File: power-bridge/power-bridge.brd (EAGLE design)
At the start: 9.8 x 22.4 mm, 3 parts, among them X2 CON-MA03-2PCB_EDGE

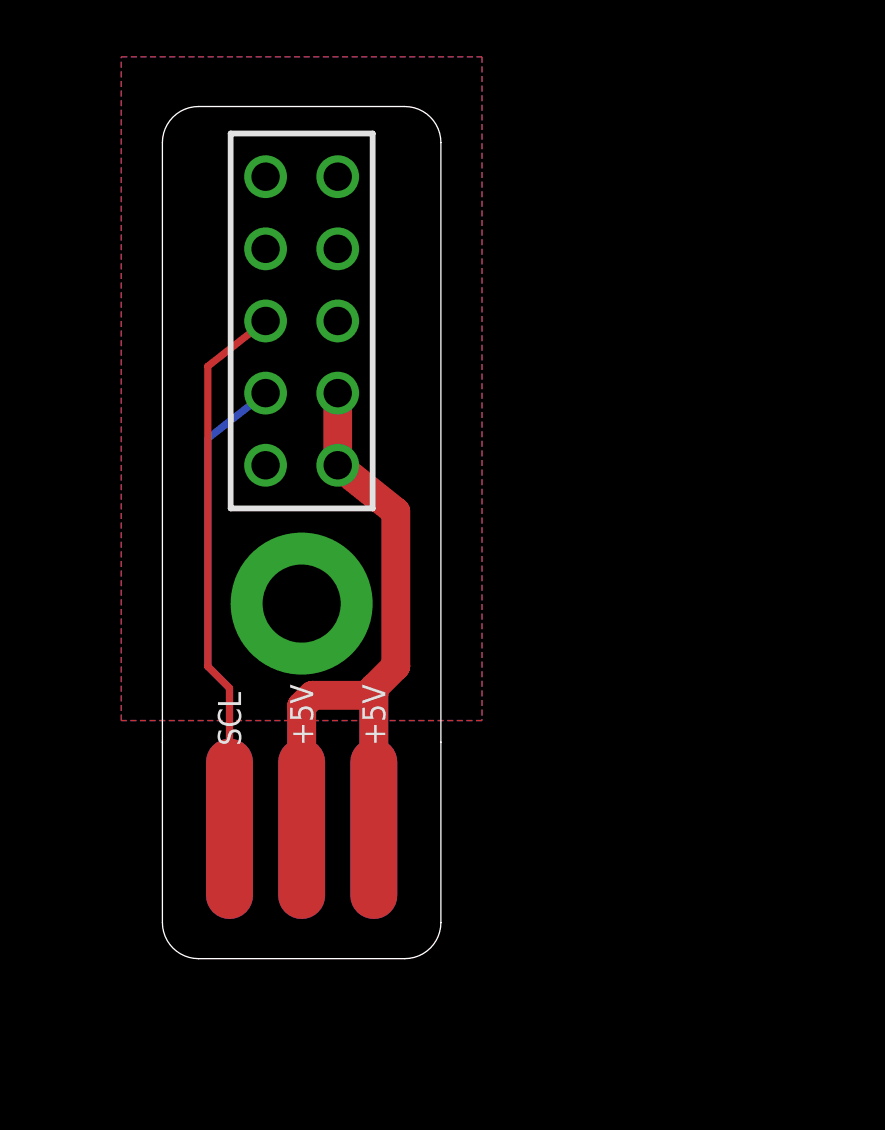
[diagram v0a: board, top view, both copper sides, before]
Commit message: Publish v1.0.0 Power Board and Power Bridge
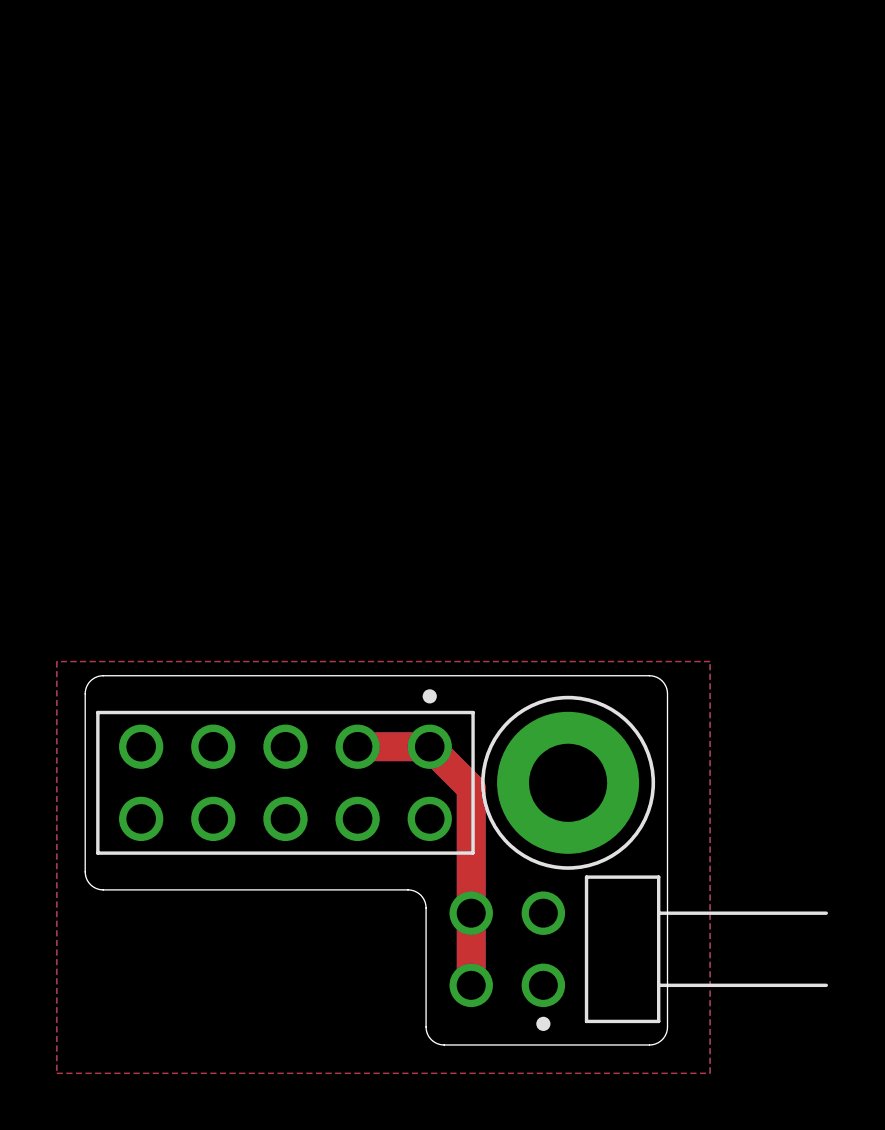
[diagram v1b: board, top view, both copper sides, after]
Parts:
- removed U$2: MOUNTINGHOLE2.7_THICK, sanisimov:MOUNTINGHOLE_2.7_PLATED_THICK
- added U$1: MOUNTINGHOLE2.7_THICK, _Library.b1f76137-4d0f-4ce2-9703-0cd83550450f.flbr:MOUNTINGHOLE_2.7_PLATED_THICK
- X1: value (none) -> CON-MA02-2; device sanisimov:FE05-2 -> _Library.b1f76137-4d0f-4ce2-9703-0cd83550450f.flbr:HDRRA4W64P254_2X2_508X254X556B
- X2: value CON-MA03-2PCB_EDGE -> CON-FE05-2; device sanisimov:PCB_EDGE_03-2 -> _Library.b1f76137-4d0f-4ce2-9703-0cd83550450f.flbr:HDRVR10W64P254_2X5_1270X508X850B
- moved X1 24.9 mm to (16.1, 1.60)
- moved X2 8.72 mm to (12.1, 10.0), turned to 180 degrees
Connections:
- removed net N$1: X1.3, X2.4
- removed net N$2: X1.5, X2.1
- removed net PWR: X1.2, X1.4, X2.2, X2.3
- new net +5V: X1.2, X1.4, X2.1, X2.3
- net GND: now also X1.1, X1.3, X2.10; no longer X1.6, X1.9, X2.6
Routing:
- net PWR: track 23.7 -> 0.00 mm
- net +5V: track 0.00 -> 23.1 mm
- net N$2: track 19.2 -> 0.00 mm
- net N$1: track 16.6 -> 0.00 mm
- net GND: track 9.27 -> 0.00 mm
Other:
- board size 9.8 x 22.4 mm -> 20.5 x 13 mm
- board text removed: "+5V"
- board text removed: "GND"
- board text removed: "SCL"
- board text removed: "SDA"
